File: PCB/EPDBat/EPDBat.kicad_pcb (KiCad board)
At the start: 4 copper layers, 70 x 70 mm, 50 parts, among them J1 Conn_01x26, J10 JST-PH-SM3-TB, J4 Conn_01x02, J5 TC2030-USB-NL-DS, J7 USB-C-Socket-V, Q1 BSS138, Q2 CJ2301, Q3 C179347, U1 TP4054, U2 ME6211C33M5G-N, U4 ESP32-S3-MINI-1

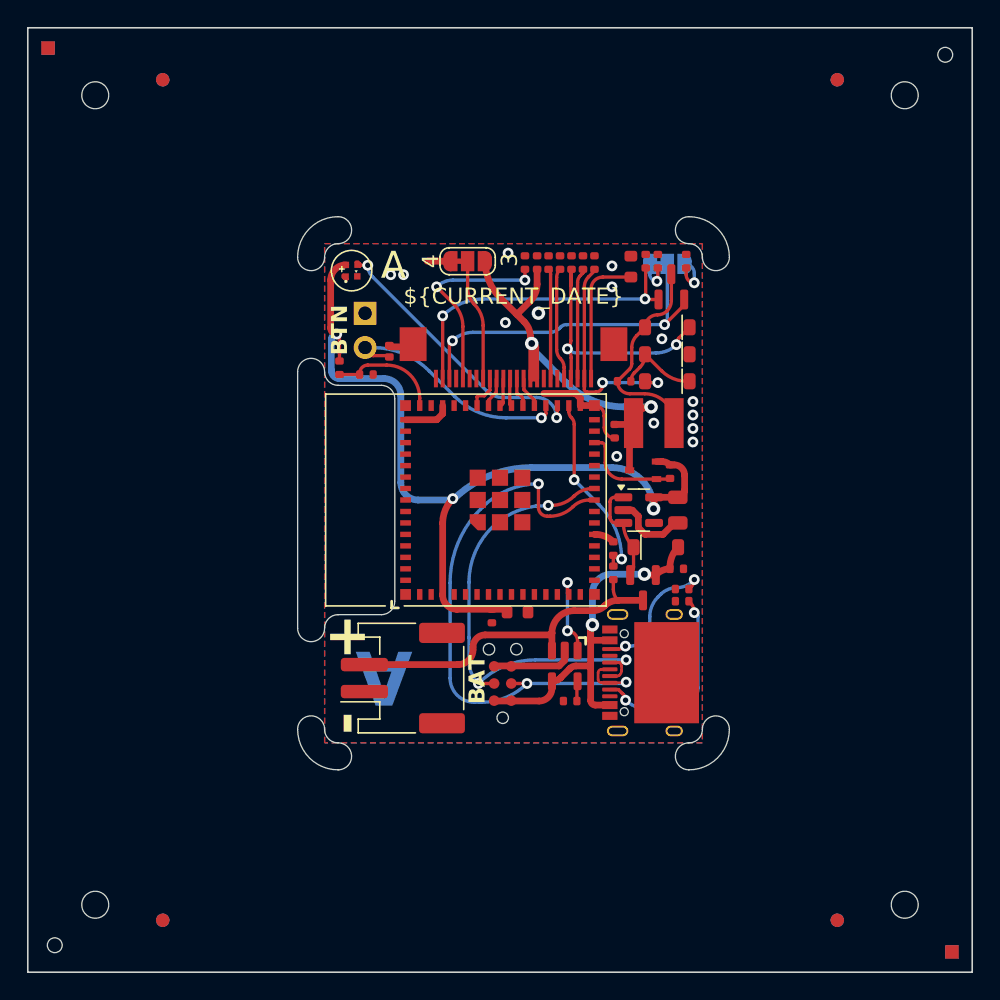
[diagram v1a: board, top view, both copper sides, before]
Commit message: PCB Update
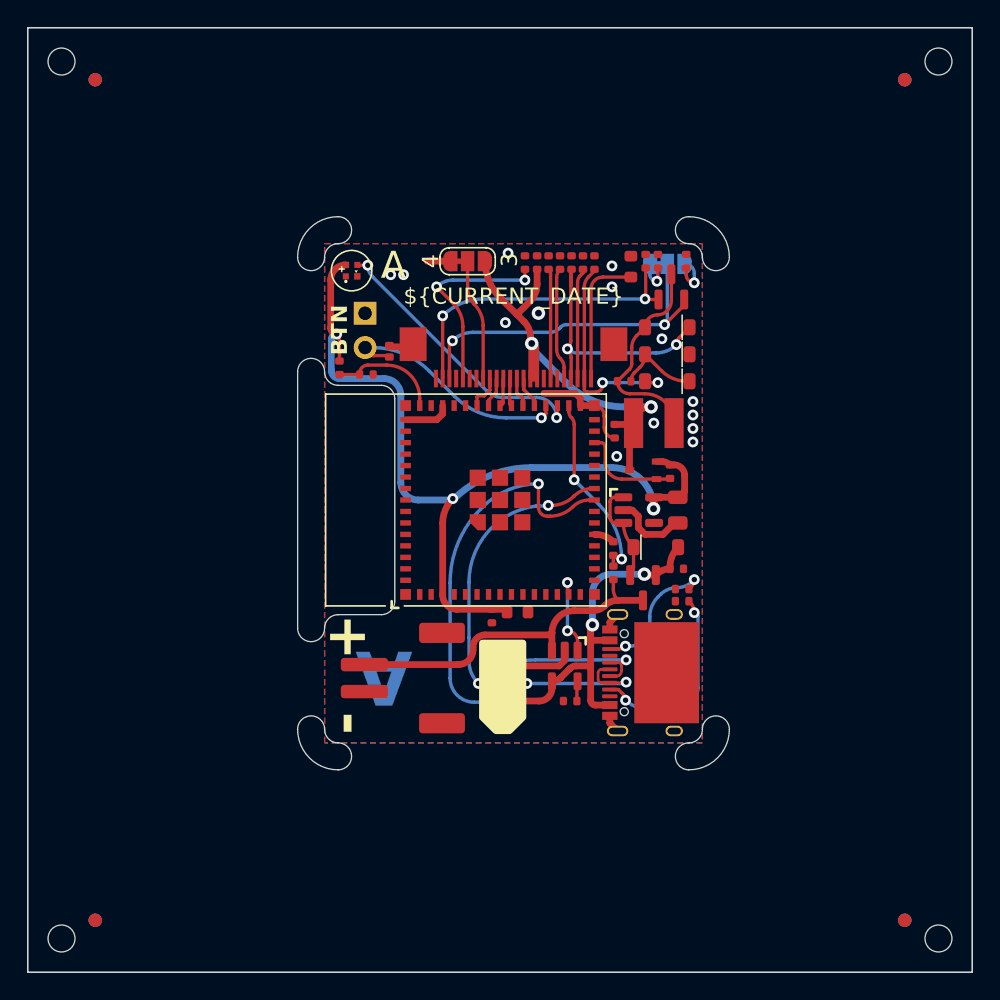
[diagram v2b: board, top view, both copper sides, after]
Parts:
- J10: footprint Connector_JST:JST_PH_S2B-PH-SM4-TB_1x02-1MP_P2.00mm_Horizontal -> RevK:JST_PH_S2B-PH-SM4-TB_1x02-1MP_P2.00mm_Horizontal
- U2: footprint Package_TO_SOT_SMD:SOT-23-5 -> RevK:SOT-23-5-90
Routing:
- net GND: track 27.5 -> 30.2 mm
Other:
- board text removed: "BAT"
